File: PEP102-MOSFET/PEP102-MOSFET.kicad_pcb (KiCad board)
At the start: 2 copper layers, 45 x 45 mm, 13 parts, among them J1 Screw_Terminal_01x02, J3 Conn_01x02_Pin, J4 Conn_01x02_Pin, J5 Conn_01x02_Pin, J6 Conn_01x02_Pin, Q19 2N7002

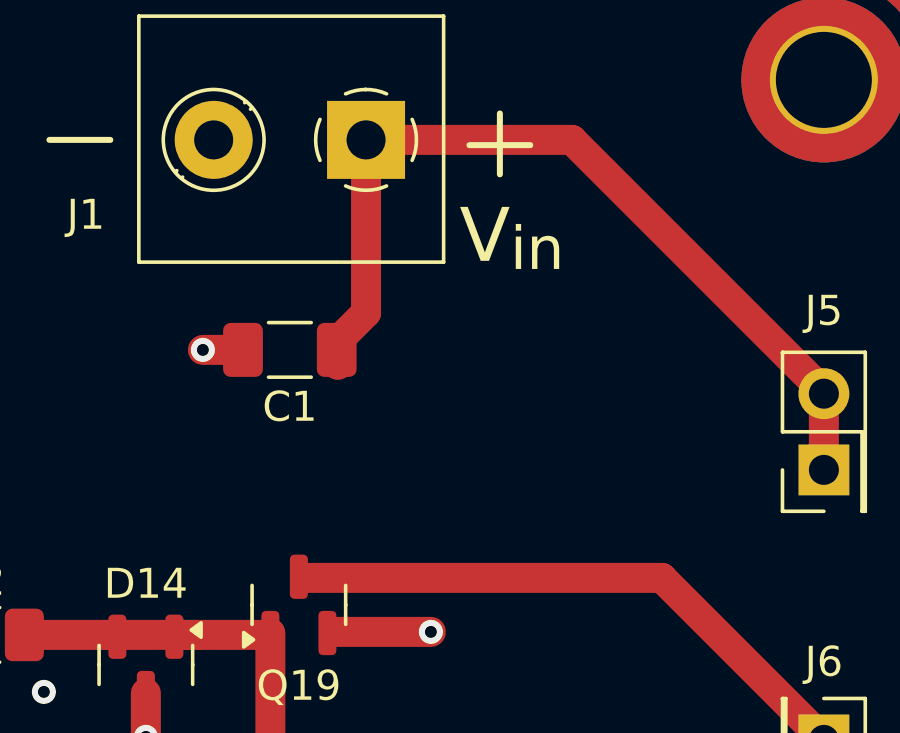
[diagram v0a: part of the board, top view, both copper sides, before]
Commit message: Nova estetika.
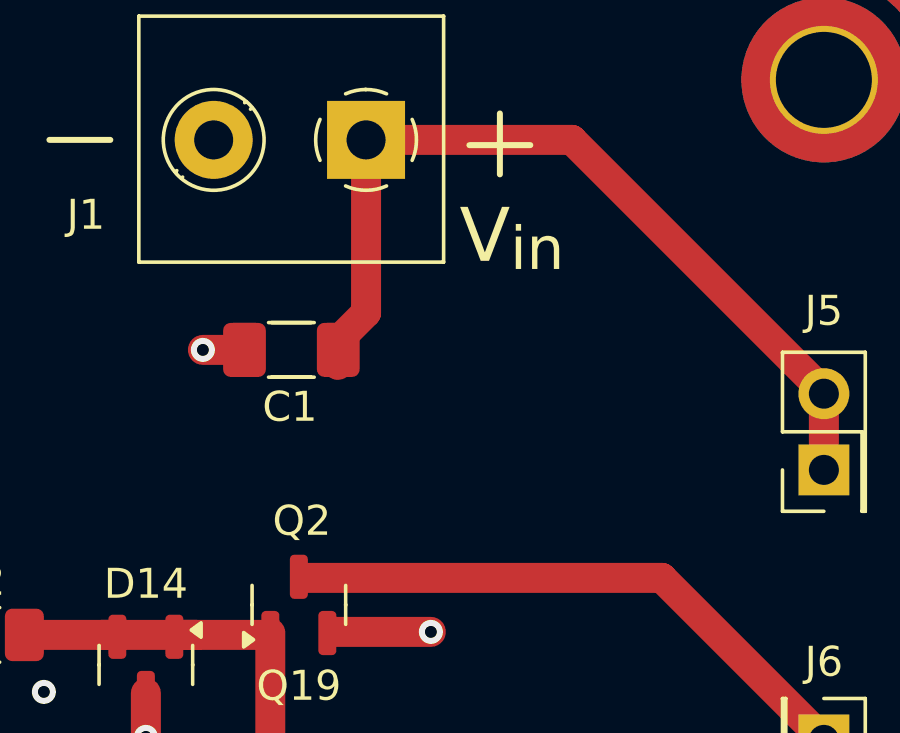
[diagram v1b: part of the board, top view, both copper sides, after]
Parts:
- added C1: 100n, Capacitor_SMD:C_1206_3216Metric_Pad1.33x1.80mm_HandSolder, F.Cu at (122.3, 114.0)
- added REF**: R_silk_symbol, PEP_library:R_silk_symbol, F.Cu at (110.0, 116.7)
- added REF**: zener_silk, PEP_library:zener_silk, F.Cu at (122.3, 133.4)
- added REF**: C_silk_symbol, PEP_library:C_silk_symbol, F.Cu at (125.3, 118.8)
- added REF**: NMOS_silk, PEP_library:NMOS_silk, F.Cu at (123.8, 131.4)
- added REF**: zener_silk, PEP_library:zener_silk, F.Cu at (119.3, 133.4)
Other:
- board text added: "Q2"
- board text removed: "V_{drain}"
